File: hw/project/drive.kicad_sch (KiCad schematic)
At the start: 63 parts, among them Q10 STL110N10F7, Q5 STL110N10F7, Q6 STL110N10F7, Q7 STL110N10F7, Q8 STL110N10F7, Q9 STL110N10F7

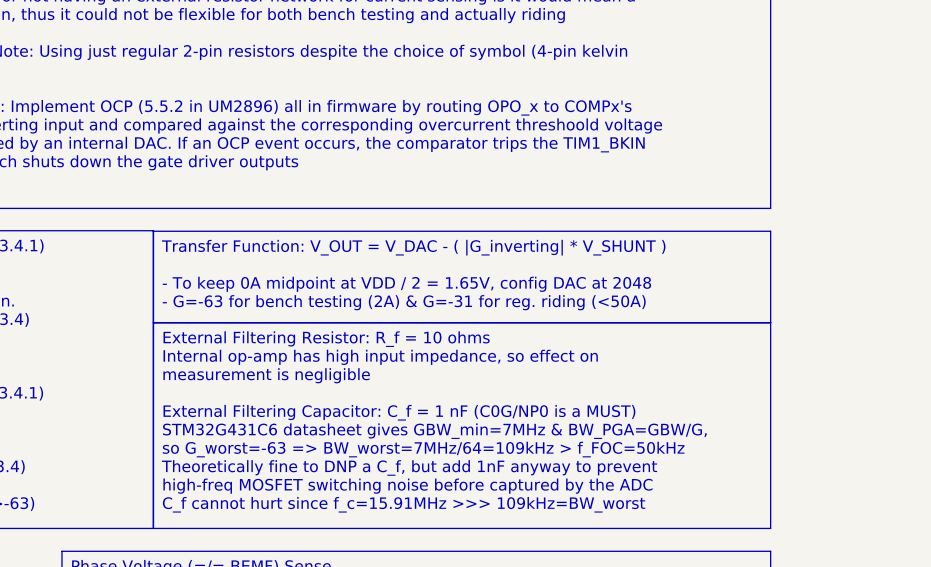
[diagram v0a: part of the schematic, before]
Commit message: Prep to revamp power sheet
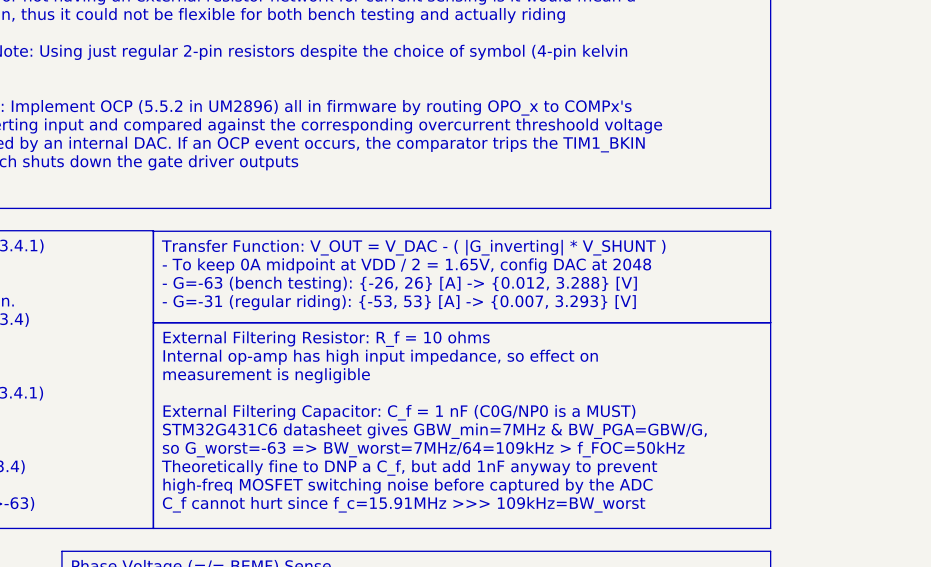
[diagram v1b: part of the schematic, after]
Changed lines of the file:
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@@
 		)
 	)
-	(text_box "Transfer Function: V_OUT = V_DAC - ( |G_inverting| * V_SHUNT )\n\n- To keep 0A midpoint at VDD / 2 = 1.65V, config DAC at 2048\n- G=-63 for bench testing (2A) & G=-31 for reg. riding (<50A)"
+	(text_box "Transfer Function: V_OUT = V_DAC - ( |G_inverting| * V_SHUNT )\n- To keep 0A midpoint at VDD / 2 = 1.65V, config DAC at 2048\n- G=-63 (bench testing): {-26, 26} [A] -> {0.012, 3.288} [V]\n- G=-31 (regular riding): {-53, 53} [A] -> {0.007, 3.293} [V]"
 		(exclude_from_sim no)
 		(at 246.38 109.2201 0)
